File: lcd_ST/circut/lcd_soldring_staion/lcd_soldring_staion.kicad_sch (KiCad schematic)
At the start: 28 parts, among them J1 DIN-5, J1 Screw_Terminal_01x02, J2 Conn_01x05_Pin, J3 Conn_01x01_Pin, J4 Conn_01x01_Pin, J5 Conn_01x01_Pin, J6 Conn_01x01_Pin, J7 Conn_01x04_Pin, Q1 IRF7403, SW1 SW_Push, U1 PIC16F15223T-I/SL, U2 L7805, U3 LM358

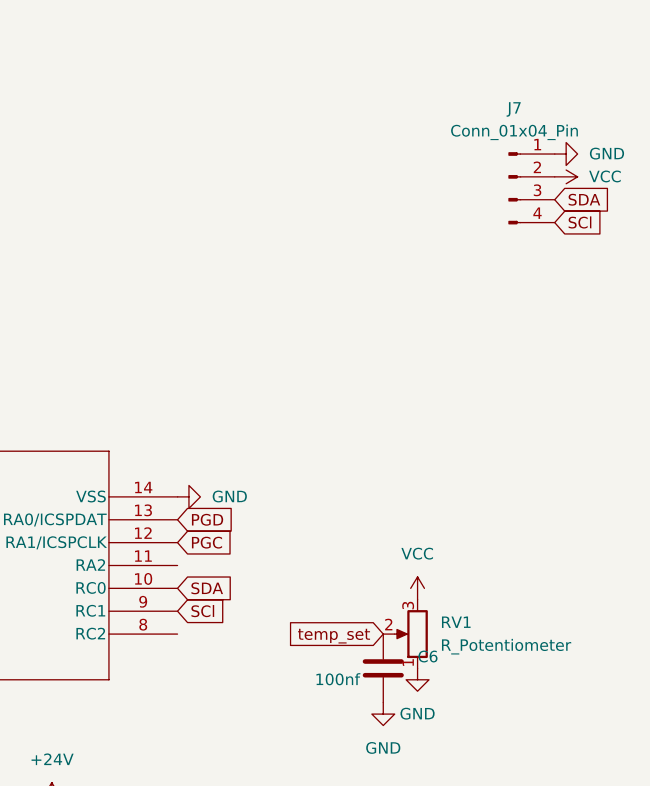
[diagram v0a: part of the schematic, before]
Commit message: Update lcd_soldring_staion.kicad_sch
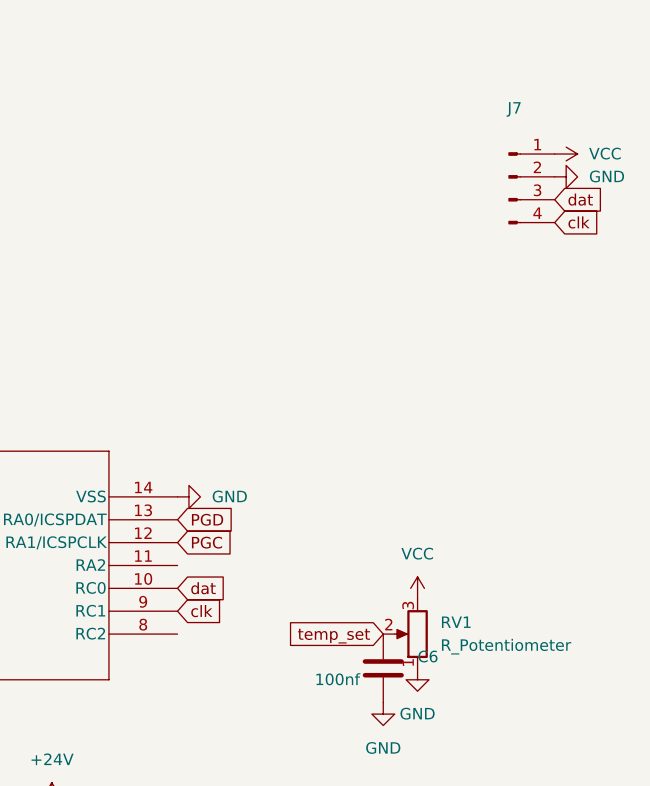
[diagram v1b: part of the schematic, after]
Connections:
- net GND: now also J7.2 (Pin_2); no longer J7.1 (Pin_1)
- net VCC: now also J7.1 (Pin_1); no longer J7.2 (Pin_2)
- net SCl renamed clk
- net SDA renamed dat
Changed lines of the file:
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@@
 		)
 	)
-	(global_label "SDA"
+	(global_label "dat"
 		(shape input)
 		(at 274.32 40.64 0)
@@
 		)
 		(property "Intersheetrefs" "${INTERSHEET_REFS}"
-			(at 280.8733 40.64 0)
+			(at 280.3289 40.64 0)
 			(effects
 				(font
@@
 		)
 	)
-	(global_label "SDA"
-		(shape input)
-		(at 232.41 83.82 0)
-		(fields_autoplaced yes)
-		(effects
-			(font
-				(size 1.27 1.27)
-			)
-			(justify left)
-		)
-		(property "Intersheetrefs" "${INTERSHEET_REFS}"
-			(at 238.9633 83.82 0)
-			(effects
-				(font
-					(size 1.27 1.27)
-				)
-				(justify left)
-				(hide yes)
-			)
-		)
-	)
 	(global_label "heater_gate"
 		(shape input)
@@
 		)
 	)
+	(global_label "clk"
+		(shape input)
+		(at 232.41 86.36 0)
+		(fields_autoplaced yes)
+		(effects
+			(font
+				(size 1.27 1.27)
+			)
+			(justify left)
+		)
+		(property "Intersheetrefs" "${INTERSHEET_REFS}"
+			(at 238.1771 86.36 0)
+			(effects
+				(font
+					(size 1.27 1.27)
+				)
+				(justify left)
+				(hide yes)
+			)
+		)
+	)
 	(global_label "T+"
 		(shape input)
@@
 		)
 	)
-	(global_label "SCl"
-		(shape input)
-		(at 232.41 86.36 0)
-		(fields_autoplaced yes)
-		(effects
-			(font
-				(size 1.27 1.27)
-			)
-			(justify left)
-		)
-		(property "Intersheetrefs" "${INTERSHEET_REFS}"
-			(at 238.5399 86.36 0)
-			(effects
-				(font
-					(size 1.27 1.27)
-				)
-				(justify left)
-				(hide yes)
-			)
-		)
-	)
 	(global_label "heater"
 		(shape input)
@@
 		)
 	)
-	(global_label "SCl"
+	(global_label "clk"
 		(shape input)
 		(at 274.32 43.18 0)
@@
 		)
 		(property "Intersheetrefs" "${INTERSHEET_REFS}"
-			(at 280.4499 43.18 0)
+			(at 280.0871 43.18 0)
 			(effects
 				(font
@@
 		)
 	)
+	(global_label "dat"
+		(shape input)
+		(at 232.41 83.82 0)
+		(fields_autoplaced yes)
+		(effects
+			(font
+				(size 1.27 1.27)
+			)
+			(justify left)
+		)
+		(property "Intersheetrefs" "${INTERSHEET_REFS}"
+			(at 238.4189 83.82 0)
+			(effects
+				(font
+					(size 1.27 1.27)
+				)
+				(justify left)
+				(hide yes)
+			)
+		)
+	)
 	(global_label "PGD"
 		(shape input)
@@
 	(symbol
 		(lib_id "power:GND")
-		(at 274.32 35.56 90)
+		(at 274.32 38.1 90)
 		(unit 1)
 		(exclude_from_sim no)
@@
 		(fields_autoplaced yes)
 		(property "Reference" "#PWR019"
-			(at 280.67 35.56 0)
+			(at 280.67 38.1 0)
 			(effects
 				(font
@@
 		)
 		(property "Value" "GND"
-			(at 278.13 35.5599 90)
+			(at 278.13 38.0999 90)
 			(effects
 				(font
@@
 		)
 		(property "Footprint" ""
-			(at 274.32 35.56 0)
+			(at 274.32 38.1 0)
 			(effects
 				(font
@@
 		)
 		(property "Datasheet" ""
-			(at 274.32 35.56 0)
+			(at 274.32 38.1 0)
 			(effects
 				(font
@@
 		)
 		(property "Description" "Power symbol creates a global label with name \"GND\" , ground"
-			(at 274.32 35.56 0)
+			(at 274.32 38.1 0)
 			(effects
 				(font
@@
 					(size 1.27 1.27)
 				)
+				(hide yes)
 			)
 		)
@@
 	(symbol
 		(lib_id "power:VCC")
-		(at 274.32 38.1 270)
+		(at 274.32 35.56 270)
 		(unit 1)
 		(exclude_from_sim no)
@@
 		(fields_autoplaced yes)
 		(property "Reference" "#PWR018"
-			(at 270.51 38.1 0)
+			(at 270.51 35.56 0)
 			(effects
 				(font
@@
 		)
 		(property "Value" "VCC"
-			(at 278.13 38.0999 90)
+			(at 278.13 35.5599 90)
 			(effects
 				(font
@@
 		)
 		(property "Footprint" ""
-			(at 274.32 38.1 0)
+			(at 274.32 35.56 0)
 			(effects
 				(font
@@
 		)
 		(property "Datasheet" ""
-			(at 274.32 38.1 0)
+			(at 274.32 35.56 0)
 			(effects
 				(font
@@
 		)
 		(property "Description" "Power symbol creates a global label with name \"VCC\""
-			(at 274.32 38.1 0)
+			(at 274.32 35.56 0)
 			(effects
 				(font

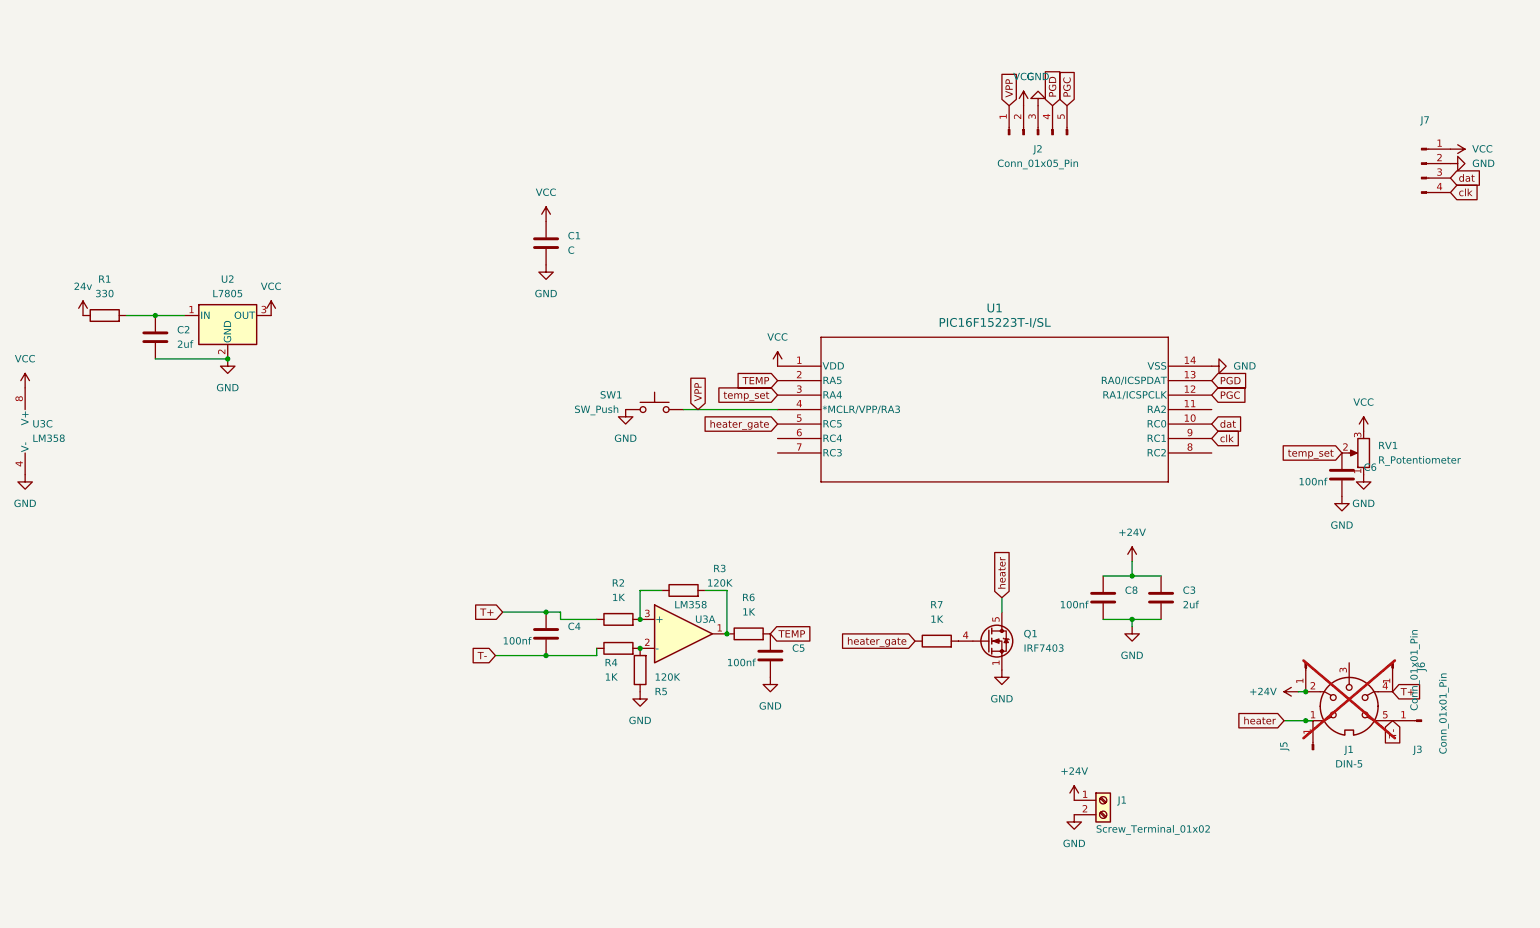
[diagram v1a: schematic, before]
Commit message: k
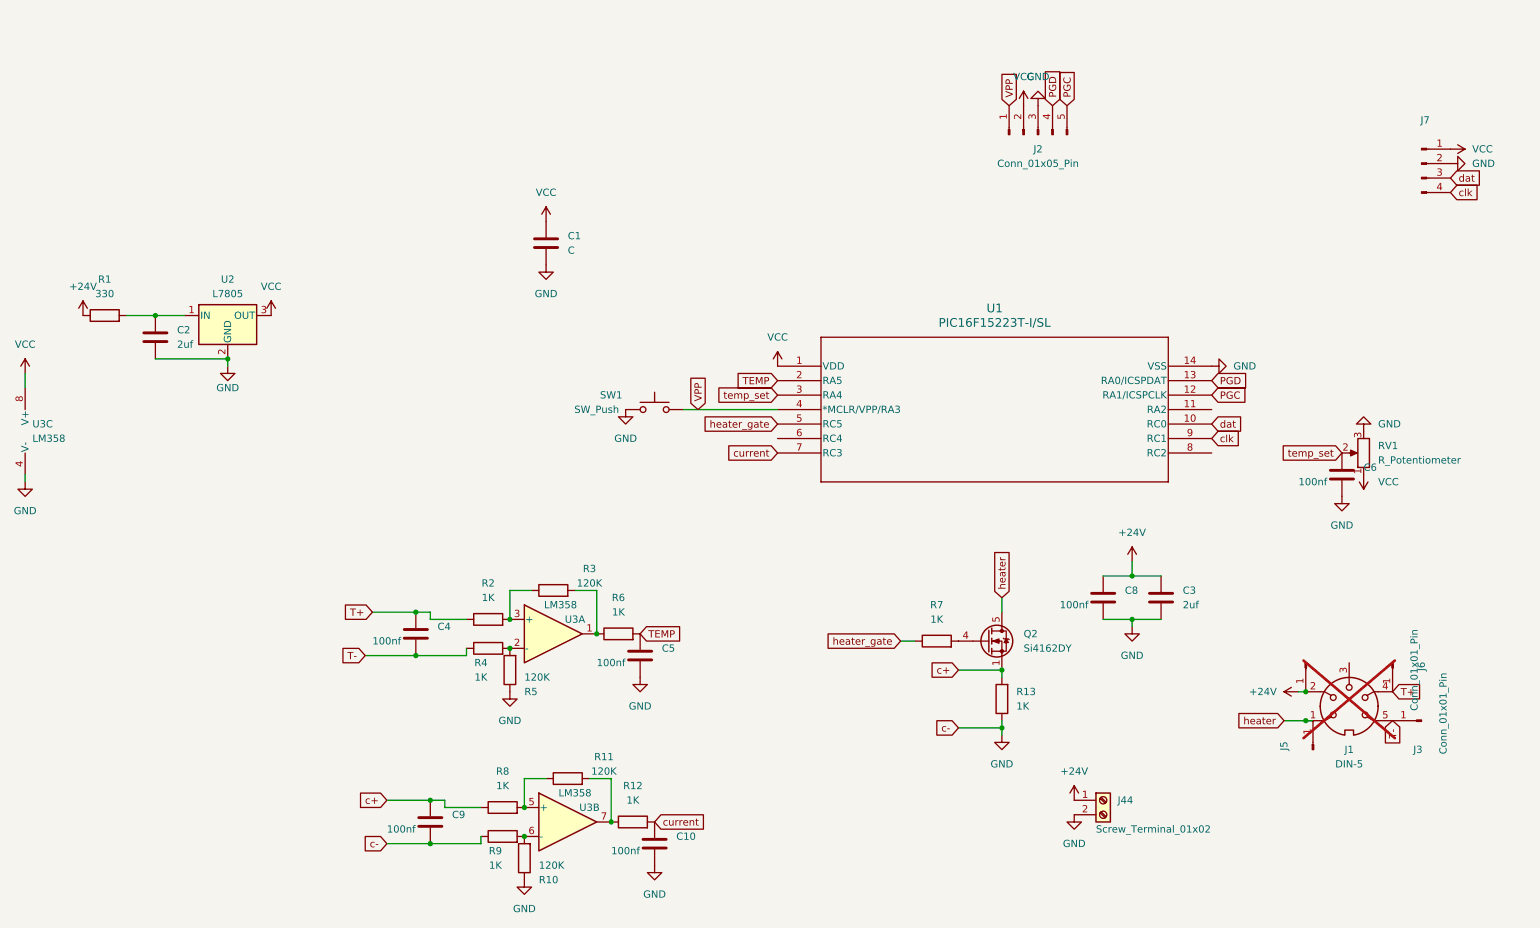
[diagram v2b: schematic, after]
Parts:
- removed Q1: IRF7403, Package_TO_SOT_SMD:Infineon_PG-HSOF-8-3_ThermalVias, symbol Transistor_FET:IRF7403
- added C10, C9: 100nf, Capacitor_SMD:C_1206_3216Metric_Pad1.33x1.80mm_HandSolder, symbol Device:C
- added Q2: Si4162DY, Package_SO:SOIC-8_3.9x4.9mm_P1.27mm, symbol Transistor_FET:Si4162DY
- added R10, R11: 120K, Resistor_SMD:R_1206_3216Metric_Pad1.30x1.75mm_HandSolder, symbol Device:R
- added R12, R8, R9: 1K, Resistor_SMD:R_1206_3216Metric_Pad1.30x1.75mm_HandSolder, symbol Device:R
- added R13: 1K, Resistor_SMD:R_1812_4532Metric_Pad1.30x3.40mm_HandSolder, symbol Device:R
- added unit 2 of U3
- C1: footprint (none) -> Capacitor_SMD:C_1206_3216Metric_Pad1.33x1.80mm_HandSolder
- J2: footprint (none) -> Connector_Molex:Molex_KK-254_AE-6410-05A_1x05_P2.54mm_Vertical
- J3: footprint Connector_JST:JST_XH_B1B-XH-AM_1x01_P2.50mm_Vertical -> Connector_PinHeader_2.54mm:PinHeader_1x01_P2.54mm_Vertical
- J4, J5, J6: footprint Connector_PinHeader_2.54mm:PinHeader_1x01_P2.54mm_Horizontal -> Connector_PinHeader_2.54mm:PinHeader_1x01_P2.54mm_Vertical
- J7: footprint (none) -> Connector:FanPinHeader_1x04_P2.54mm_Vertical
- R1, R2, R3, R4, R5, R6, R7: footprint (none) -> Resistor_SMD:R_1206_3216Metric_Pad1.30x1.75mm_HandSolder
- RV1: footprint (none) -> Potentiometer_THT:Potentiometer_ACP_CA9-H2,5_Horizontal
- SW1: footprint (none) -> Button_Switch_SMD:SW_DIP_SPSTx01_Slide_6.7x4.1mm_W6.73mm_P2.54mm_LowProfile_JPin
- U1: footprint SOIC14_SL_MCH -> pic16f15223:SOIC14_SL_MCH
- U2: footprint (none) -> Package_TO_SOT_SMD:TO-252-3_TabPin2
- U3: footprint (none) -> Package_SO:SOIC-8_5.3x6.2mm_P1.27mm
- renumbered J1 to J44
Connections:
- net 24v is gone; now on net +24V: R1.1
- net GND: now also RV1.3, C10.2, C9.2, R10.1, R13.1, R9.1; no longer RV1.1
- net VCC: now also RV1.1; no longer RV1.3
- net heater: now also Q2.5 (D), Q2.6 (D), Q2.7 (D), Q2.8 (D)
- net at R7.2: now also Q2.4 (G)
- net current: now reaches U1.7 (RC3)
- net current: now also C10.1, R12.2
- new net: R11.1, R8.2, U3.5 (+)
- new net: R10.2, R9.2, U3.6 (-)
- new net: R11.2, R12.1, U3.7
- new net c+: C9.1, Q2.1 (S), Q2.2 (S), Q2.3 (S), R13.2, R8.1
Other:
- moved on the sheet: C4, C5, R2, R3, R4, R5, R6, U3A

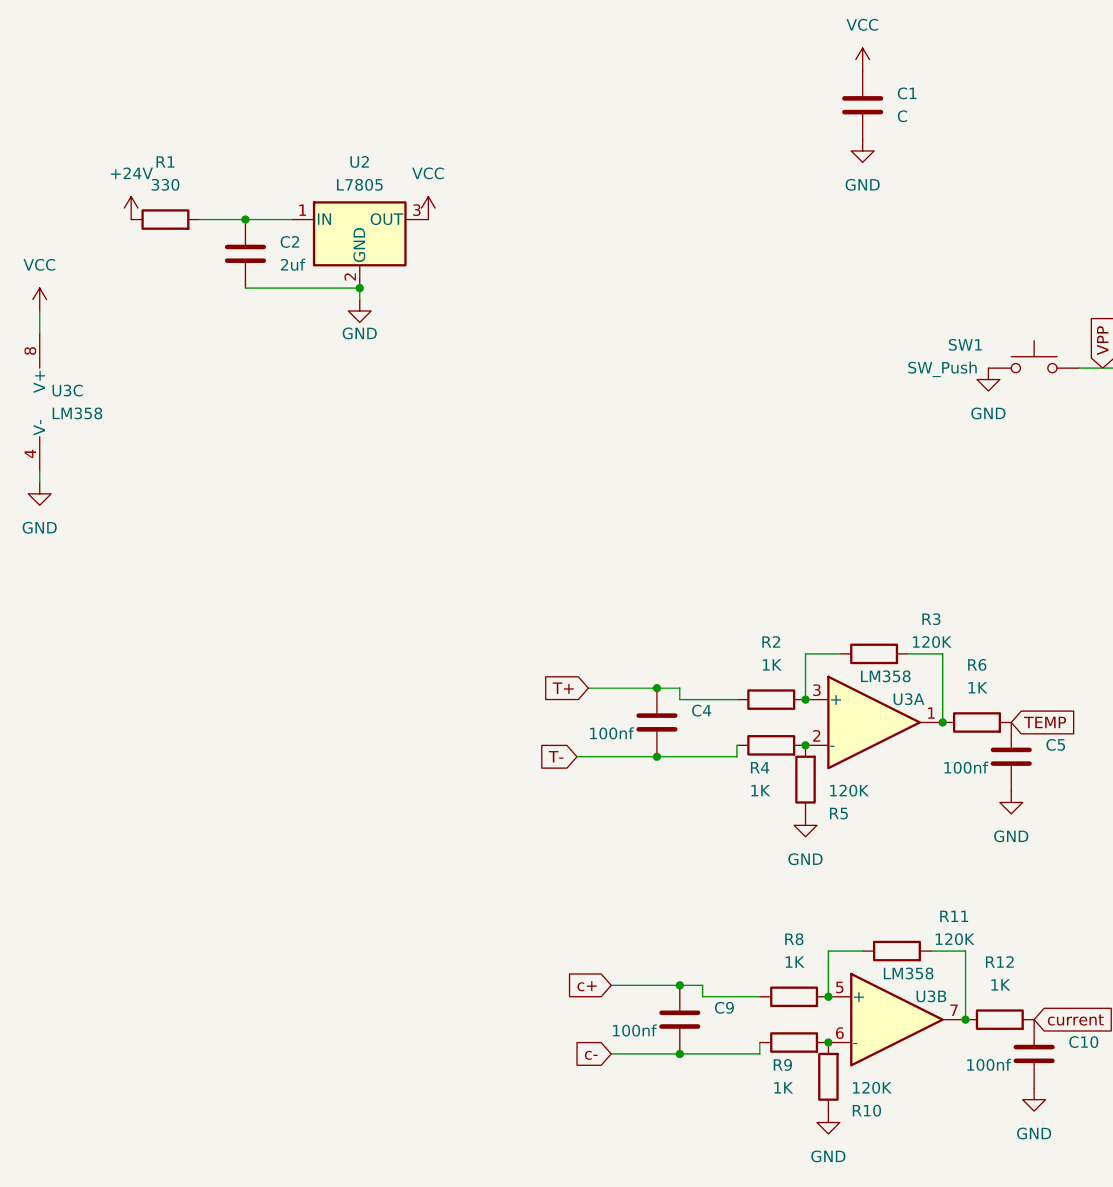
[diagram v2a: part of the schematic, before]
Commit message: done v0
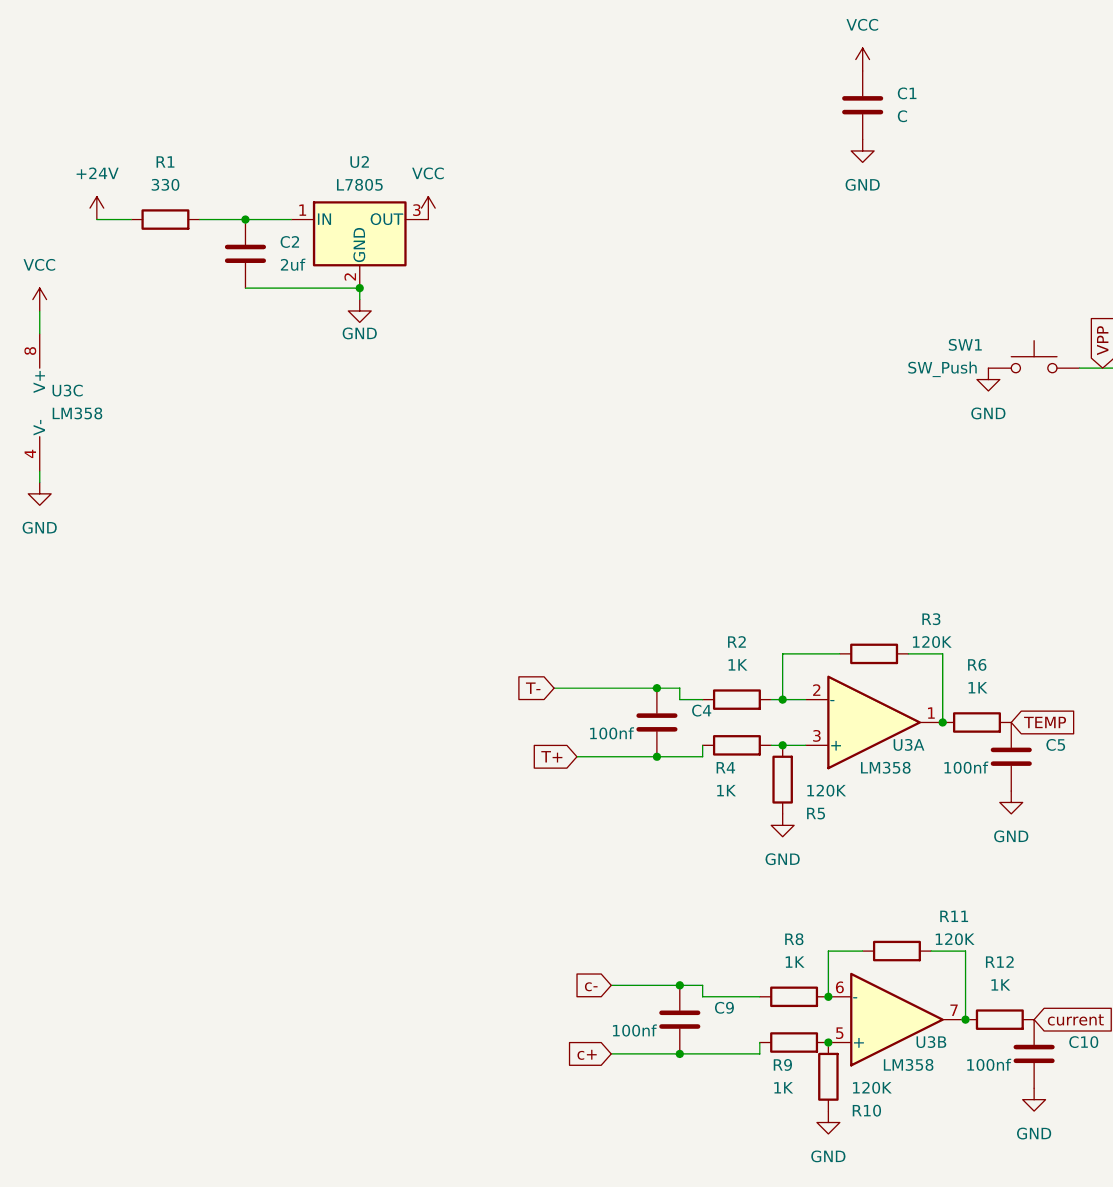
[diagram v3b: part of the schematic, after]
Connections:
- net GND: now also C9.1, R8.1; no longer C9.2, R9.1
- net T+: now also C4.2, R4.1; no longer C4.1, R2.1
- net T-: now also C4.1, R2.1; no longer C4.2, R4.1
- net c+: now also C9.2, R9.1; no longer C9.1, R8.1
- net at R11.1, R8.2: now also U3.6 (-); no longer U3.5 (+)
- net at R10.2, R9.2: now also U3.5 (+); no longer U3.6 (-)
- net at R4.2, R5.2: now also U3.3 (+); no longer U3.2 (-)
- net at R2.2, R3.1: now also U3.2 (-); no longer U3.3 (+)
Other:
- moved on the sheet: R2, R4, R5
